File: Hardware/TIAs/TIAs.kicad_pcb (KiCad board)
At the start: 2 copper layers, 33.5 x 33.5 mm, 16 parts, among them U1 Opamp_Dual

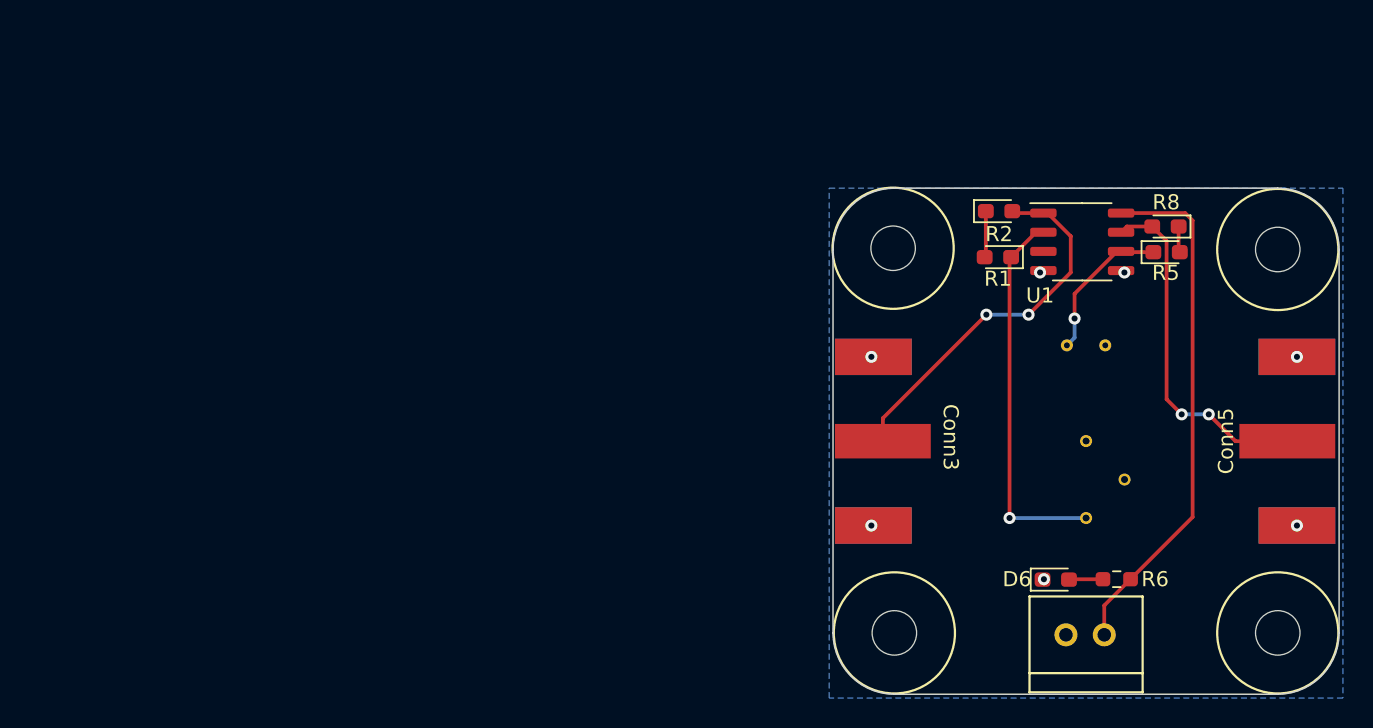
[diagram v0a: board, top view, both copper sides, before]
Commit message: Moved breakout boards to separate layouts
Edge cut no work :,(
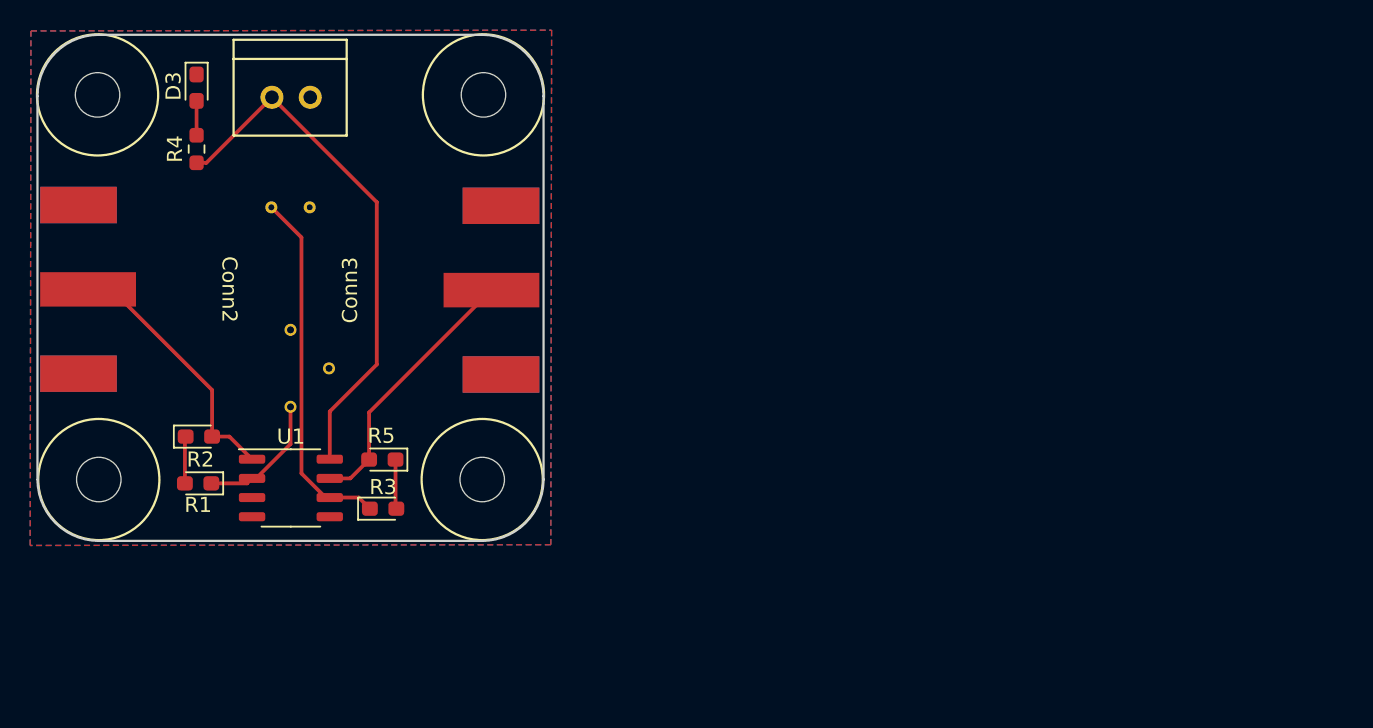
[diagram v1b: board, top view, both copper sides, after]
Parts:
- removed Conn5: PD_2, FTIR_Footprints:142-0701-801
- removed D11: S5971, FTIR_Footprints:P16113-011MN
- removed D6: Green, LED_SMD:LED_0603_1608Metric_Pad1.05x0.95mm_HandSolder
- removed H10, H11, H12, H7: MountingHole, MRDT_Drill_Holes:4_40_Hole_Corner
- removed R6: 100, Resistor_SMD:R_0603_1608Metric_Pad0.98x0.95mm_HandSolder
- removed R8: ~, LED_SMD:LED_0603_1608Metric_Pad1.05x0.95mm_HandSolder
- added Conn1: TIA, MRDT_Connectors:MOLEX_SL_02_Vertical, F.Cu at (89.6, 66.6)
- added D1: S5971, FTIR_Footprints:P16113-011MN, B.Cu at (90.8, 84.6)
- added D2: D_Photo, FTIR_Footprints:VTP9812FH, B.Cu at (90.8, 73.9)
- added H1: MountingHole, MRDT_Drill_Holes:4_40_Hole_Corner, F.Cu at (99.6, 70.5)
- added H2: MountingHole, MRDT_Drill_Holes:4_40_Hole_Corner, F.Cu at (82.0, 70.5)
- added H3: MountingHole, MRDT_Drill_Holes:4_40_Hole_Corner, F.Cu at (99.5, 87.9)
- added H4: MountingHole, MRDT_Drill_Holes:4_40_Hole_Corner, F.Cu at (82.1, 87.9)
- added R3: ~, LED_SMD:LED_0603_1608Metric_Pad1.05x0.95mm_HandSolder, F.Cu at (96.9, 93.9)
- added R4: 100, Resistor_SMD:R_0603_1608Metric_Pad0.98x0.95mm_HandSolder, F.Cu at (84.6, 70.1)
- Conn2: value TIA -> PD_1; footprint MRDT_Connectors:MOLEX_SL_02_Vertical -> FTIR_Footprints:142-0701-801
- Conn3: value PD_1 -> PD_2
- D3: value D_Photo -> Green; footprint FTIR_Footprints:VTP9812FH -> LED_SMD:LED_0603_1608Metric_Pad1.05x0.95mm_HandSolder; moved to F.Cu
- moved Conn2 71.7 mm to (76.8, 79.3), turned to -90 degrees
- moved D3 61.4 mm to (84.6, 66.0)
- moved R2 55.1 mm to (84.7, 89.1)
- moved R1 55.1 mm to (84.7, 92.2)
- moved U1 54.9 mm to (90.8, 92.5)
- moved R5 53.7 mm to (96.9, 90.6), turned to 180 degrees
- moved Conn3 26.6 mm to (104.7, 79.4), turned to 90 degrees
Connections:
- Conn2 pad 1: (no net) -> Net-(Conn2-Tip)
- Conn2 pad 2: (no net) -> GND
- Conn3 pad 1: (no net) -> Net-(Conn3-Tip)
- Conn3 pad 2: (no net) -> GND
- D3 pad 1: (no net) -> GND
- D3 pad 2: (no net) -> Net-(D3-A)
- R1 pad 1: (no net) -> Net-(D1-K)
- R1 pad 2: (no net) -> Net-(R1-Pad2)
- R2 pad 1: (no net) -> Net-(R1-Pad2)
- R2 pad 2: (no net) -> Net-(Conn2-Tip)
- R5 pad 1: (no net) -> Net-(R3-Pad2)
- R5 pad 2: (no net) -> Net-(Conn3-Tip)
- U1 pad 1: (no net) -> Net-(Conn2-Tip)
- U1 pad 2: (no net) -> Net-(D1-K)
- U1 pad 3: (no net) -> GND
- U1 pad 4: (no net) -> GND
- U1 pad 5: (no net) -> GND
- U1 pad 6: (no net) -> Net-(D2-K)
- U1 pad 7: (no net) -> Net-(Conn3-Tip)
- U1 pad 8: (no net) -> +3V3
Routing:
- net (no net): track 125.3 -> 0.00 mm, vias 13 -> 0
- net +3V3: track 0.00 -> 34.9 mm
- net Net-(D2-K): track 0.00 -> 24.0 mm
- net Net-(Conn3-Tip): track 0.00 -> 17.7 mm
- net Net-(Conn2-Tip): track 0.00 -> 17.3 mm
- net Net-(D1-K): track 0.00 -> 8.79 mm
- net Net-(R3-Pad2): track 0.00 -> 3.27 mm
- net Net-(R1-Pad2): track 0.00 -> 3.12 mm
- net Net-(D3-A): track 0.00 -> 2.28 mm
- added copper zone on B.Cu, net GND
- added copper zone on F.Cu, net GND
- removed copper zone on B.Cu, net (none)
